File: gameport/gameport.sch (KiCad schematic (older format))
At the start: 38 parts, among them J1 Conn_01x10, J2 DB15_Female, J3 X, J4 Y, J5 B1, J6 B2, U1 LDL1117S50R, U2 TL072, U3 40106, U4 555, U5 555, U6 555

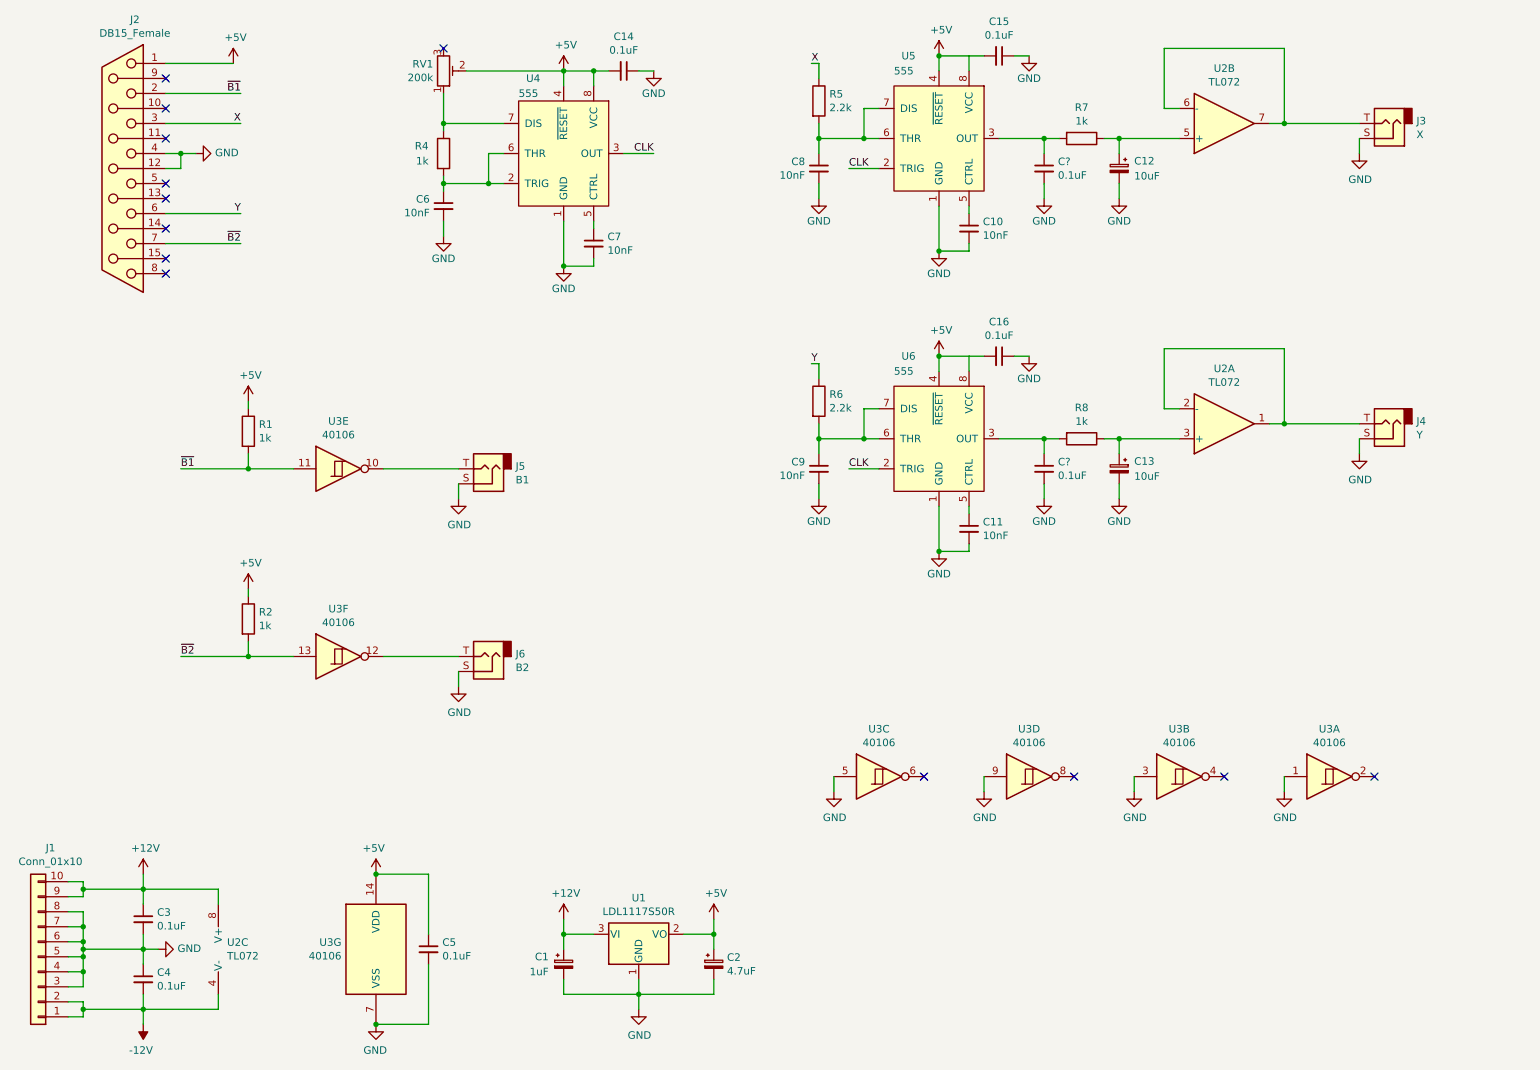
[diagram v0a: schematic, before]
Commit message: Update schematic
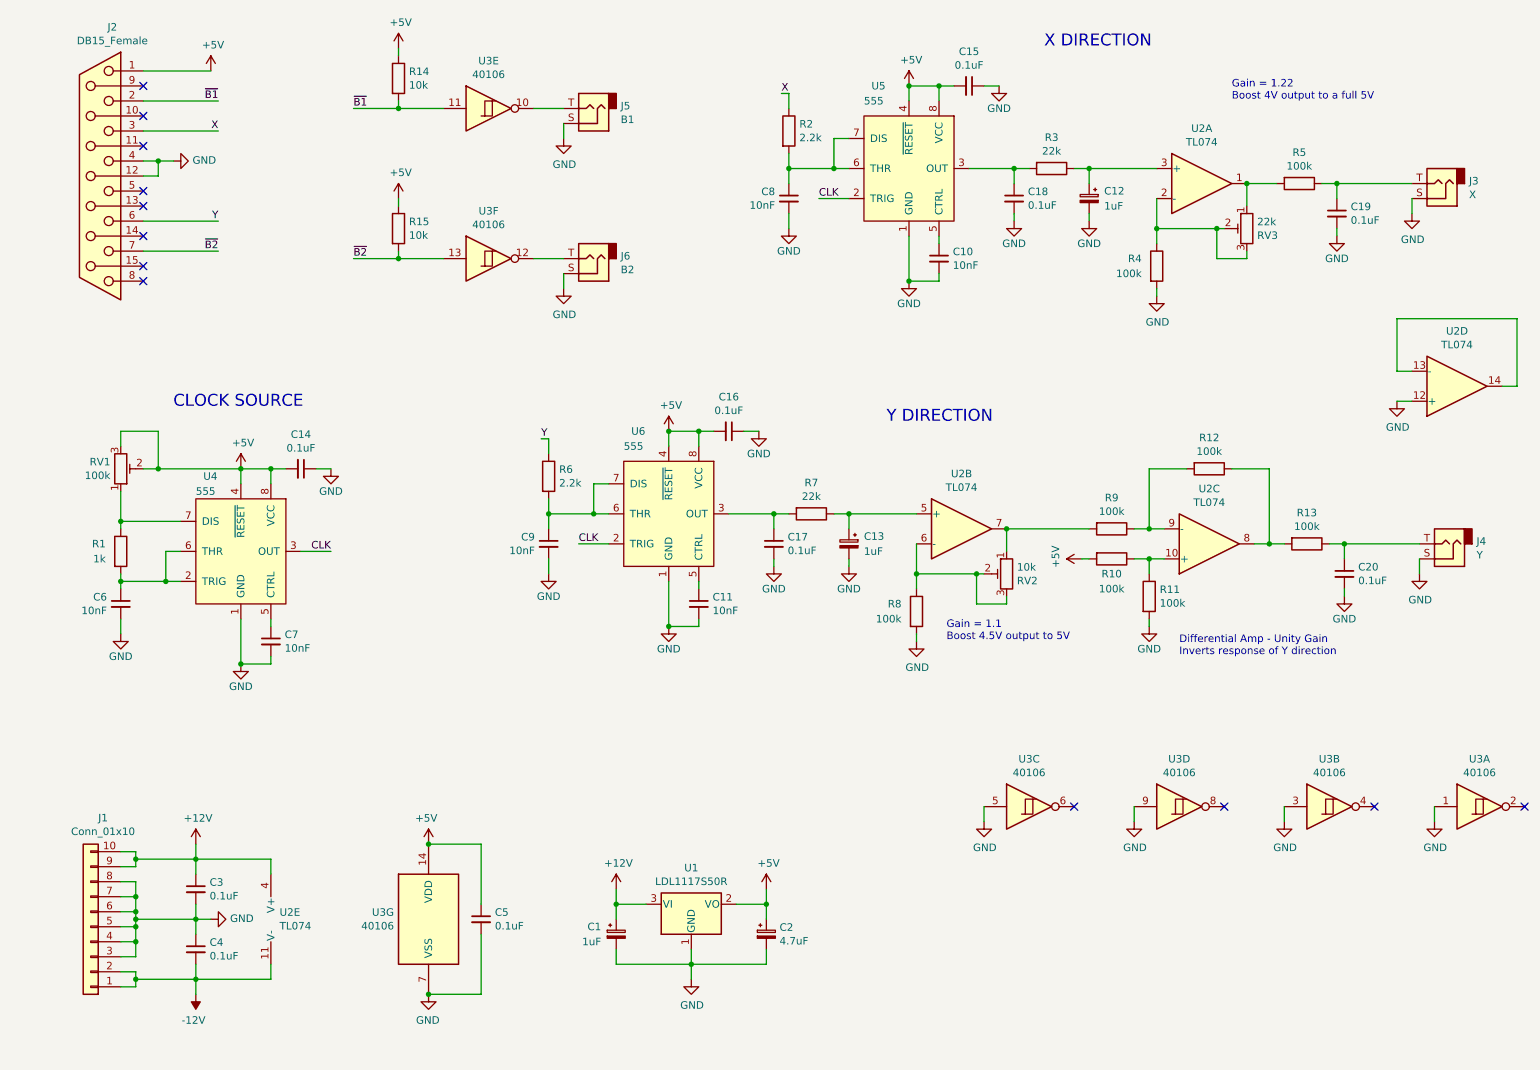
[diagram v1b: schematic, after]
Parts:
- removed U2: TL072, Package_DIP:DIP-8_W7.62mm, symbol Amplifier_Operational:TL072
- added C19, C20: 0.1uF, Capacitor_THT:C_Disc_D3.0mm_W1.6mm_P2.50mm, symbol Device:C_Small
- added R10, R11, R12, R13, R4, R5, R8, R9: 100k, Resistor_THT:R_Axial_DIN0207_L6.3mm_D2.5mm_P10.16mm_Horizontal, symbol Device:R
- added RV2: 10k, Potentiometer_THT:Potentiometer_Bourns_3296Y_Vertical, symbol Device:R_POT_TRIM
- added RV3: 22k, Potentiometer_THT:Potentiometer_Bourns_3296Y_Vertical, symbol Device:R_POT_TRIM
- added U2: TL074, Package_DIP:DIP-14_W7.62mm, symbol Amplifier_Operational:TL074
- C12, C13: value 10uF -> 1uF
- R14: renamed from R1; value 1k -> 10k
- R15: renamed from R2; value 1k -> 10k
- R3: renamed from R7; value 1k -> 22k
- R7: renamed from R8; value 1k -> 22k
- RV1: value 200k -> 100k
- gave numbers to parts that had none: 2
- renumbered R4 to R1, R5 to R2
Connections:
- net +12V: now also U2.4 (V+)
- net +5V: now also RV1.3, R10.2
- net -12V: now also U2.11 (V-)
- net GND: now also C19.2, C20.2, R11.2, R4.2, R8.2, U2.12 (+)
- net at J4.T: now also C20.1, R13.1
- net at C13.1, R7.1: now also U2.5 (+)
- net at C12.1, R3.1: now also U2.3 (+)
- net at J3.T: now also C19.1, R5.1
- new net: R5.2, RV3.1, U2.1
- new net: R4.1, RV3.2, RV3.3, U2.2 (-)
- new net: R8.1, RV2.2, RV2.3, U2.6 (-)
- new net: R9.2, RV2.1, U2.7
- new net: R10.1, R11.1, U2.10 (+)
- new net: R12.1, R13.2, U2.8
- new net: R12.2, R9.1, U2.9 (-)
- new net: U2.13 (-), U2.14
- no-connect marks 13 -> 12
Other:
- note added: "CLOCK SOURCE"
- note added: "Differential Amp - Unity Gain\nInverts response of Y direction"
- note added: "Gain = 1.1\nBoost 4.5V output to 5V"
- note added: "Gain = 1.22\nBoost 4V output to a full 5V"
- note added: "X DIRECTION"
- note added: "Y DIRECTION"
- moved on the sheet: C1, C10, C11, C12, C13, C14, C15, C16, C17, C18, C2, C3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
